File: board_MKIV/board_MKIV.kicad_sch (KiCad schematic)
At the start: 42 parts, among them J1 1757242, J2 jst-power, J3 JST -SM, J4 S3B-EH, J5 1770979, J6-Right-Angle 86094327313755E1LF, J7-Straight 86094328314755V1LF, U1 ESP32-DEVKITC-32D, U2 LTV-846S, U3 TLV272CDR, U4 BAT46W, U5 BA&

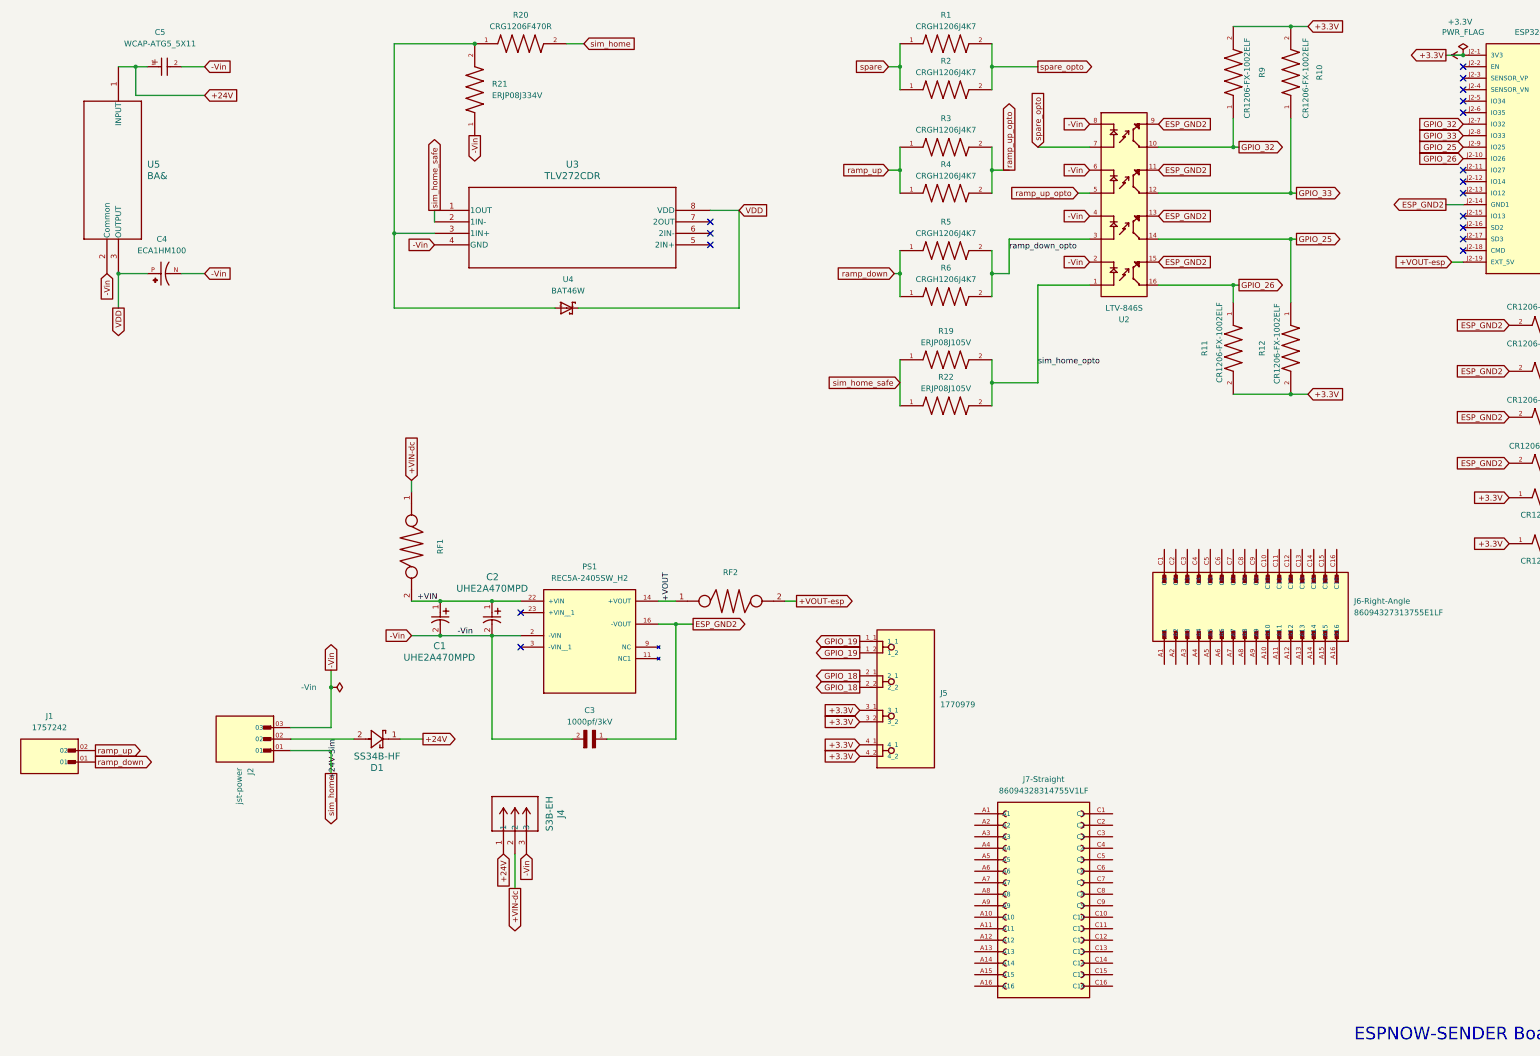
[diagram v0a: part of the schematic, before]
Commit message: update
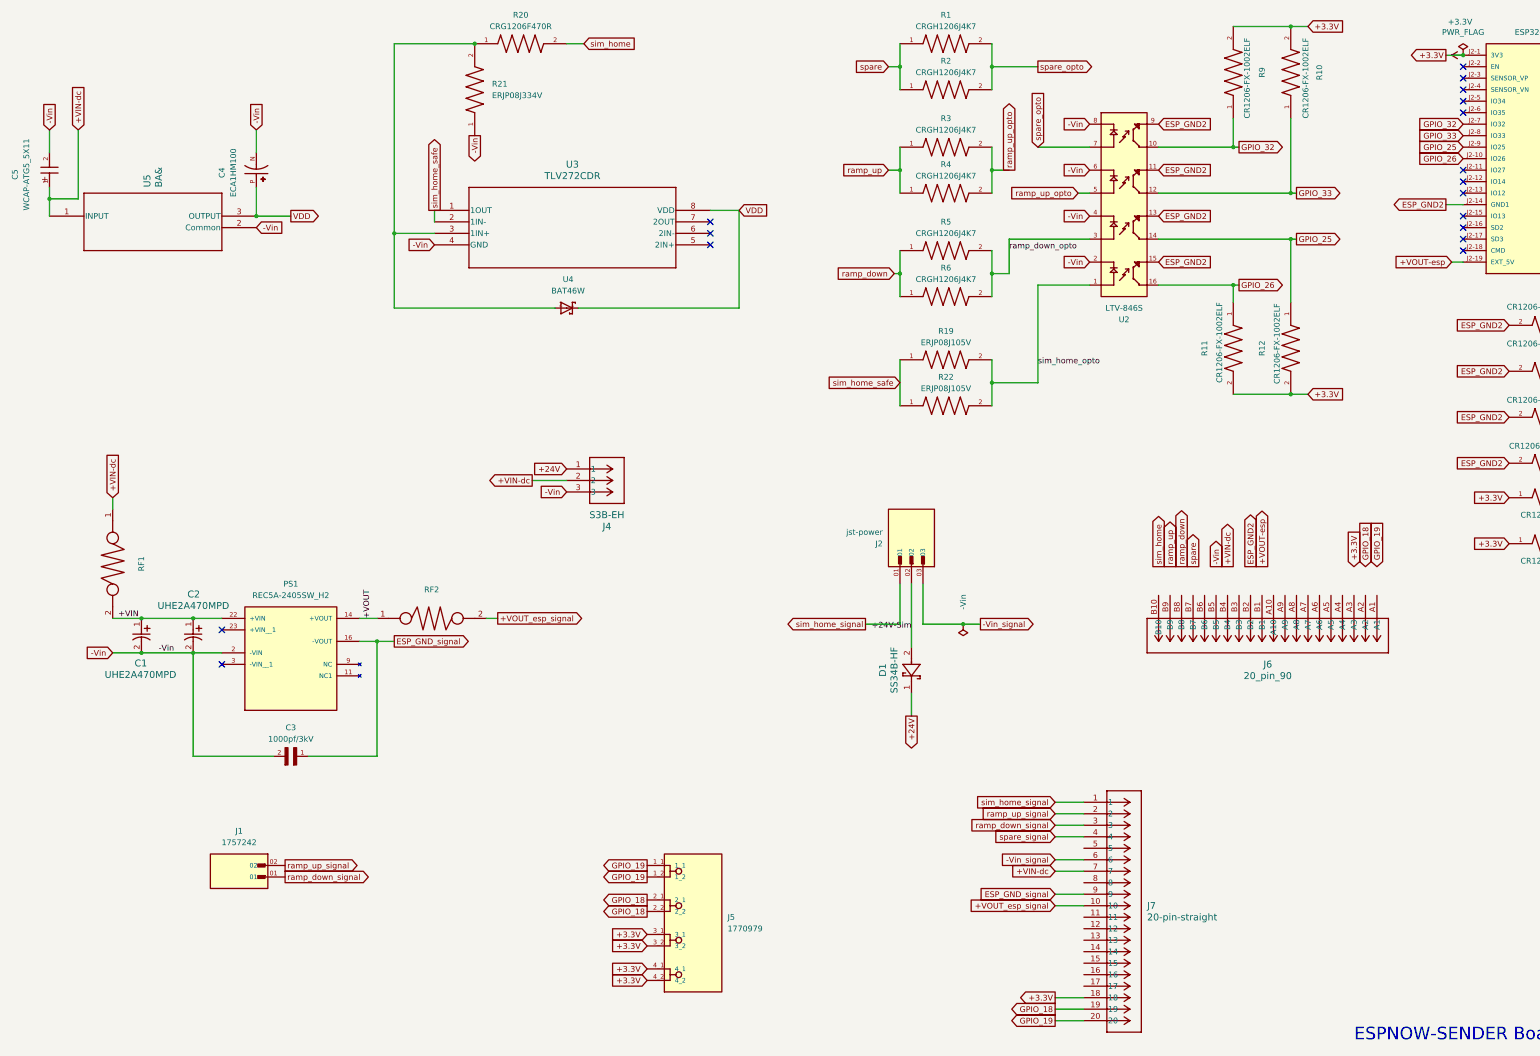
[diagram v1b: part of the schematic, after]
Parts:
- removed J6-Right-Angle: 86094327313755E1LF, 86094327313755E1LF:AMPHENOL_86094327313755E1LF, symbol 86094327313755E1LF:86094327313755E1LF
- removed J7-Straight: 86094328314755V1LF, 86094328314755V1LF:AMPHENOL_86094328314755V1LF, symbol 86094328314755V1LF:86094328314755V1LF
- added J6: 20_pin_90, CONN_XC5A-2022_OMR, symbol 20_pin_90:XC5A-2022
- added J7: 20-pin-straight, CONN_XC5B-2021_OMR, symbol 20_pin_straight:XC5B-2021
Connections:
- net +24V: no longer C5.1, U5.1 (INPUT)
- net +3.3V: now also J7.18
- net +VIN-dc: now also C5.1, U5.1 (INPUT), J7.7
- net +VOUT-esp: no longer RF2.2
- net -Vin: no longer J2.03
- net ESP_GND2: no longer C3.1, PS1.16 (-VOUT)
- net GPIO_18: now also J7.19
- net GPIO_19: now also J7.20
- net ramp_down: no longer J1.01
- net ramp_up: no longer J1.02
- net sim_home: no longer J2.01
- new net +VOUT_esp_signal: J7.10, RF2.2
- new net -Vin_signal: J2.03, J7.6
- new net ESP_GND_signal: C3.1, J7.9, PS1.16 (-VOUT)
- new net ramp_down_signal: J1.01, J7.3
- new net ramp_up_signal: J1.02, J7.2
- new net sim_home_signal: J2.01, J7.1
- new net spare_signal: J7.4
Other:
- moved on the sheet: C1, C2, C3, C4, C5, D1, J1, J2, J4, J5, PS1, RF1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
